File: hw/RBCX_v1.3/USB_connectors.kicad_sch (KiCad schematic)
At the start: 25 parts, among them J49 Conn_01x04, J50 Conn_01x04, Q15 Q_NMOS_DGS, U21 USB_C, U22 AP33772

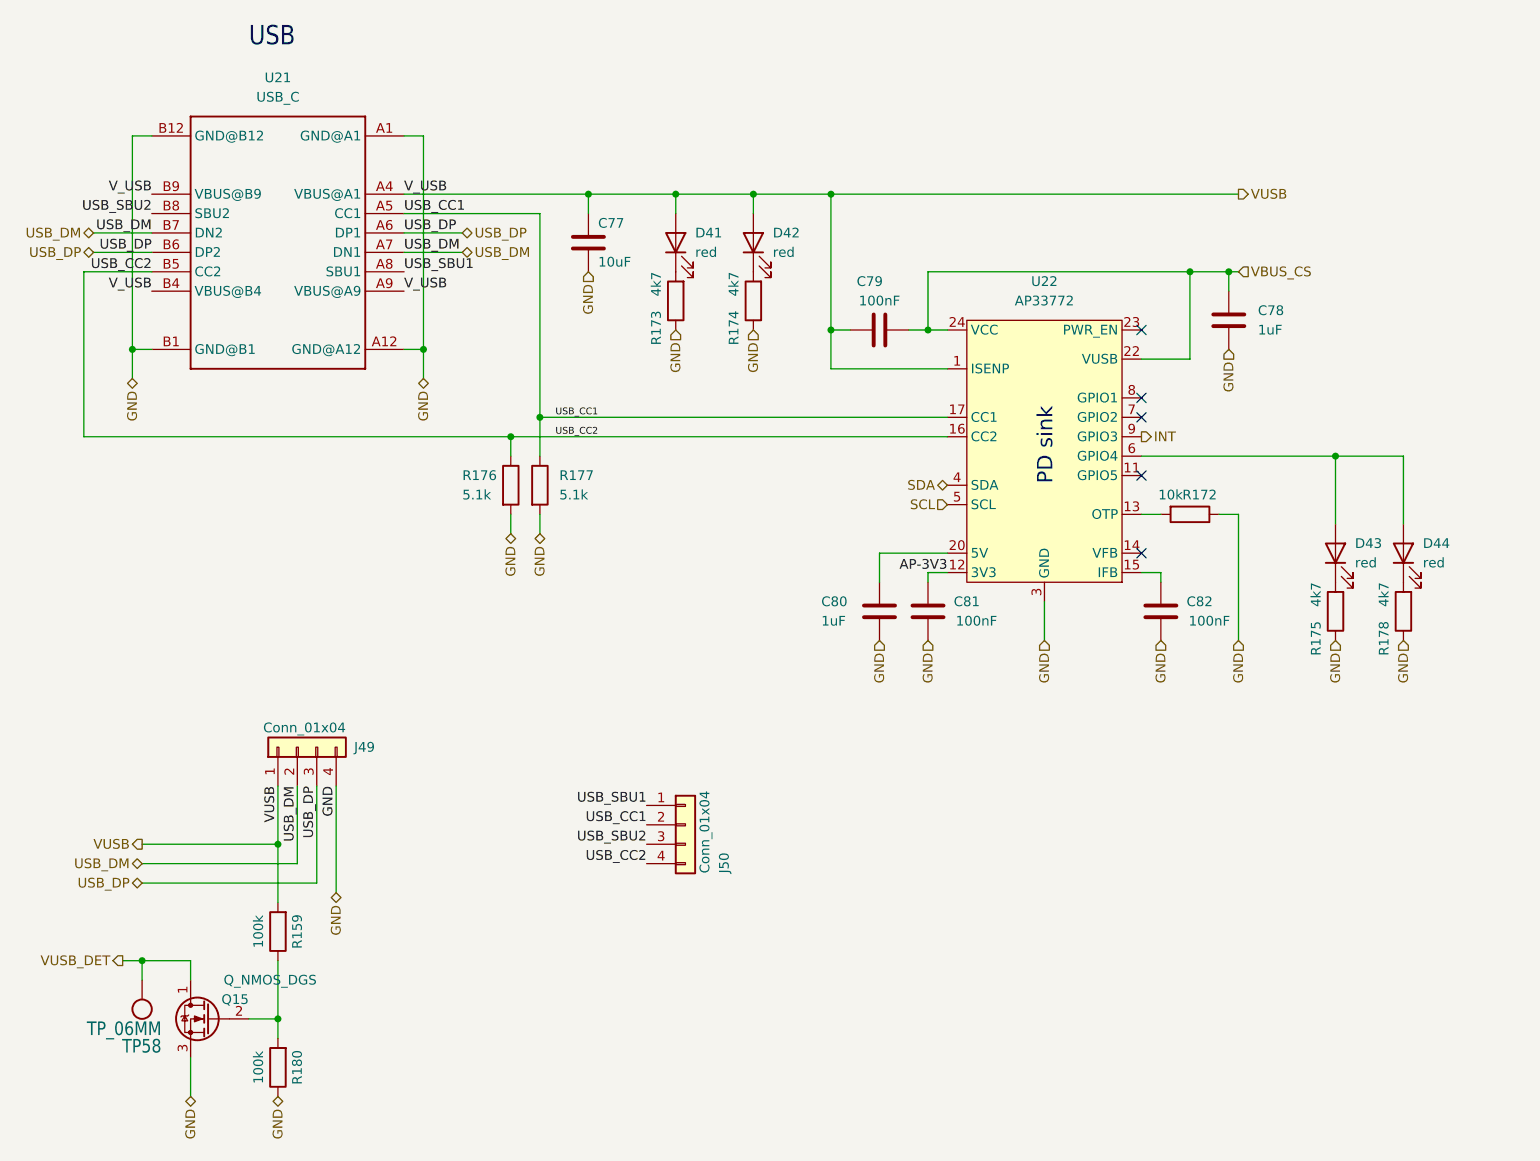
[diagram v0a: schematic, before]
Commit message: ESD and I-Servo hacker
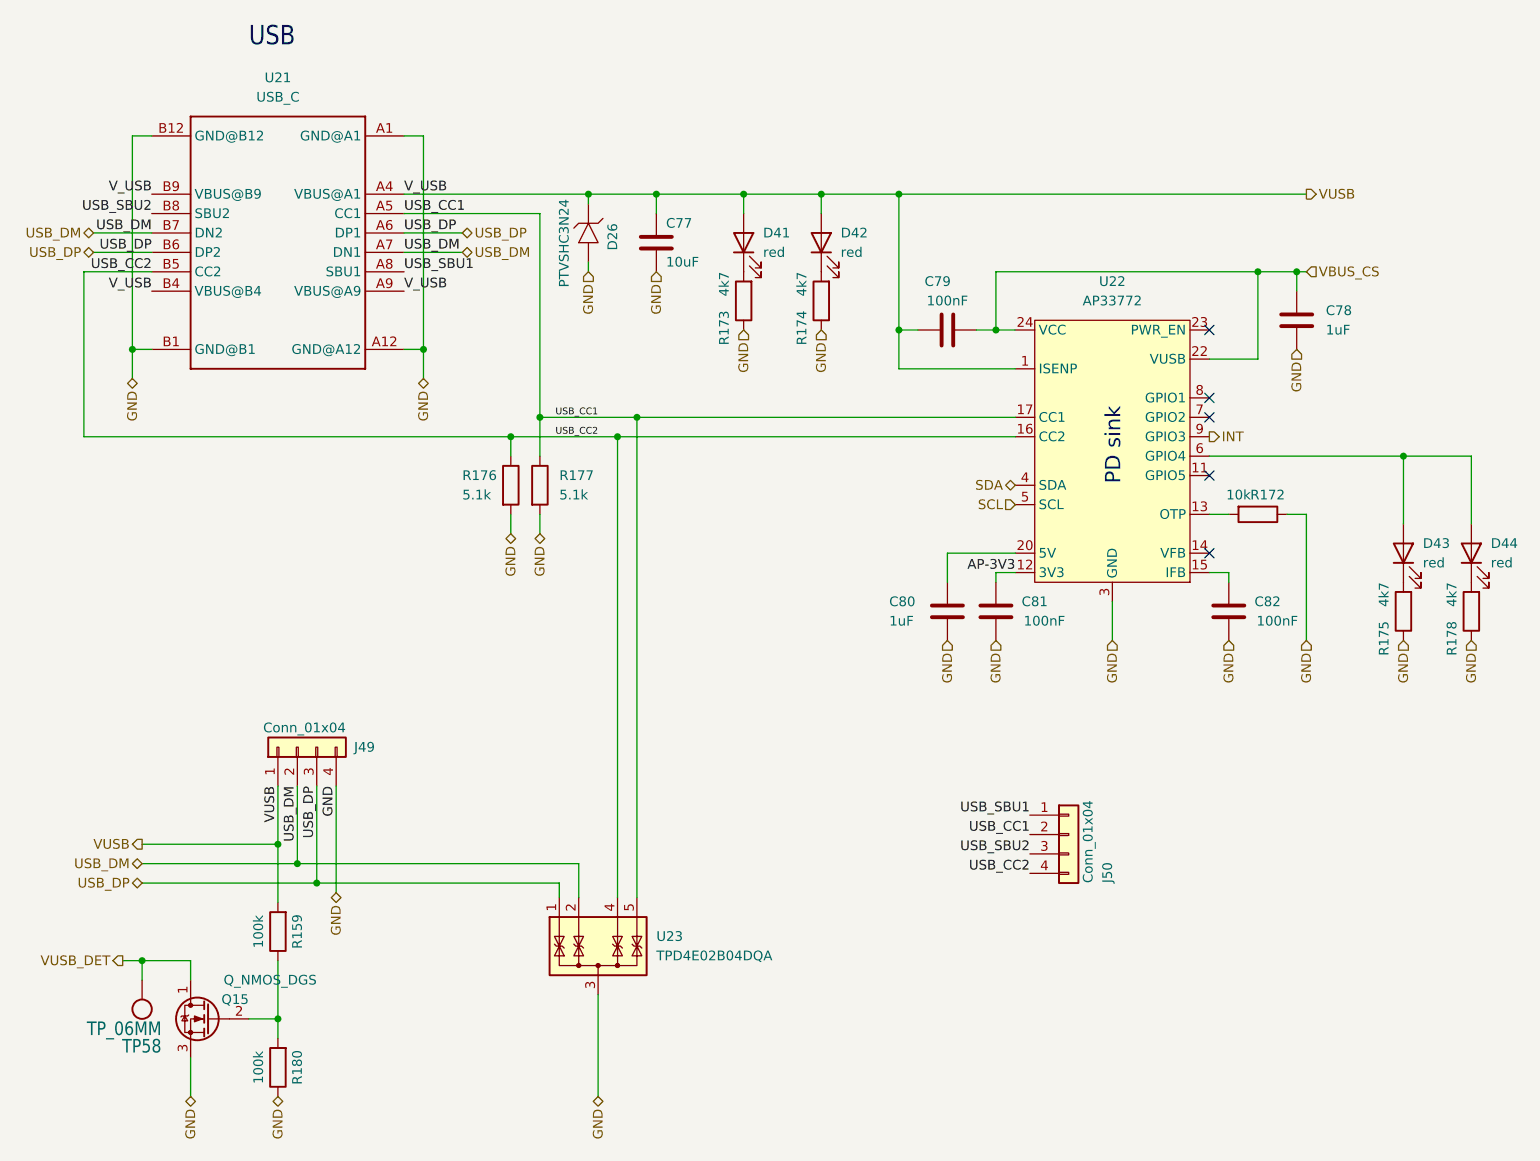
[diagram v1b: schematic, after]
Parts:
- added D26: PTVSHC3N24, Robotarna_KiCad_Library:DFN3-2x2, symbol Robotarna_KiCad_Library:PTVSHC3N24
- added U23: TPD4E02B04DQA, Package_SON:USON-10_2.5x1.0mm_P0.5mm, symbol Power_Protection:TPD4E02B04DQA
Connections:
- net GND: now also D26.1 (A), D26.2 (A), U23.3 (G), U23.8 (G)
- net USB_CC1: now also U23.5 (IO4)
- net USB_CC2: now also U23.4 (IO3)
- net USB_DM: now also U23.2 (IO2)
- net USB_DP: now also U23.1 (IO1)
- net VUSB: now also D26.3 (K)
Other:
- moved on the sheet: C77, C78, C79, C80, C81, C82, D41, D42, D43, D44, J50, R172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
